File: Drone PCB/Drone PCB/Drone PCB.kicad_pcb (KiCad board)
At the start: 2 copper layers, 46 x 60 mm, 39 parts, among them J1 Conn_01x02_Socket, J2 Conn_01x02_Socket, J3 Conn_01x02_Socket, J4 Conn_01x02_Socket, J5 Conn_01x02_Socket, J6 Conn_01x02_Socket, J7 Conn_01x06_Socket, Q1 SI2302, Q2 SI2302, Q3 SI2302, Q4 SI2302, SW1 SW_SPDT, SW2 SW_Push, U1 AMS1117-3.3, U2 ATmega328P-A, U3 MPU-9250, U4 NRF24, Y1 16MHz

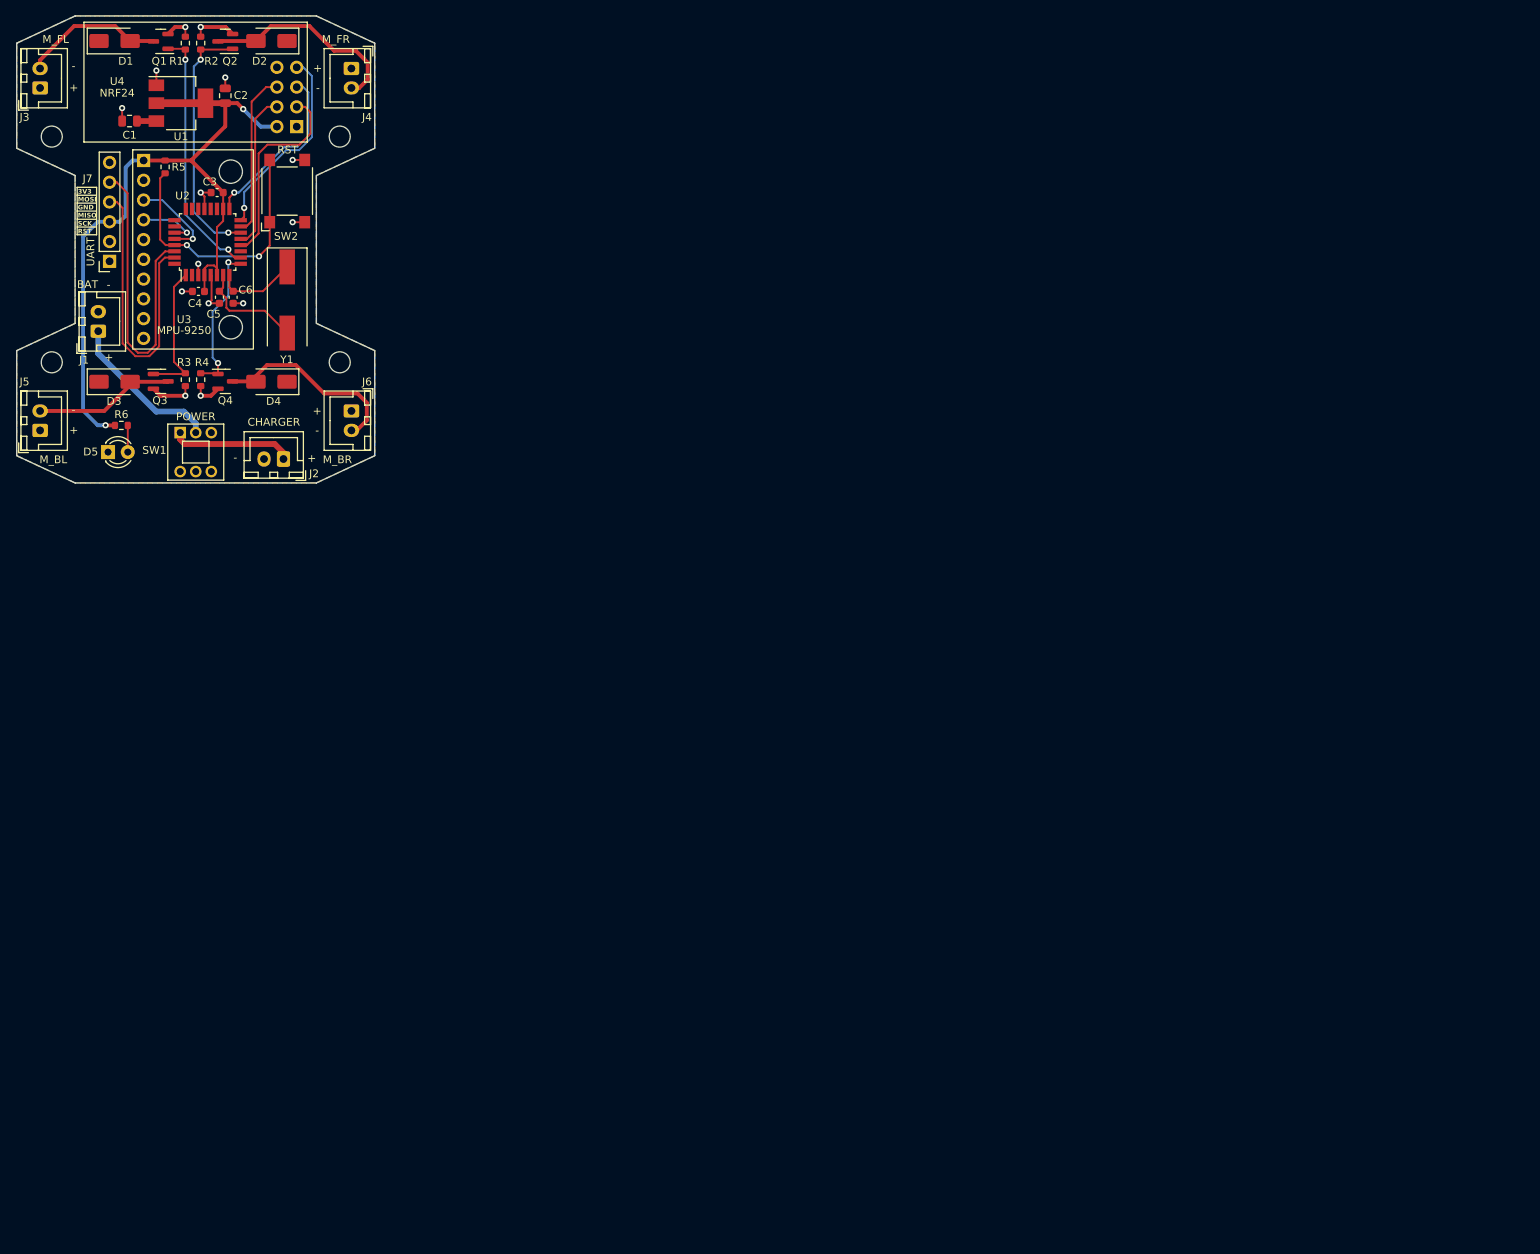
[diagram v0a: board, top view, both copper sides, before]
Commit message: Images included
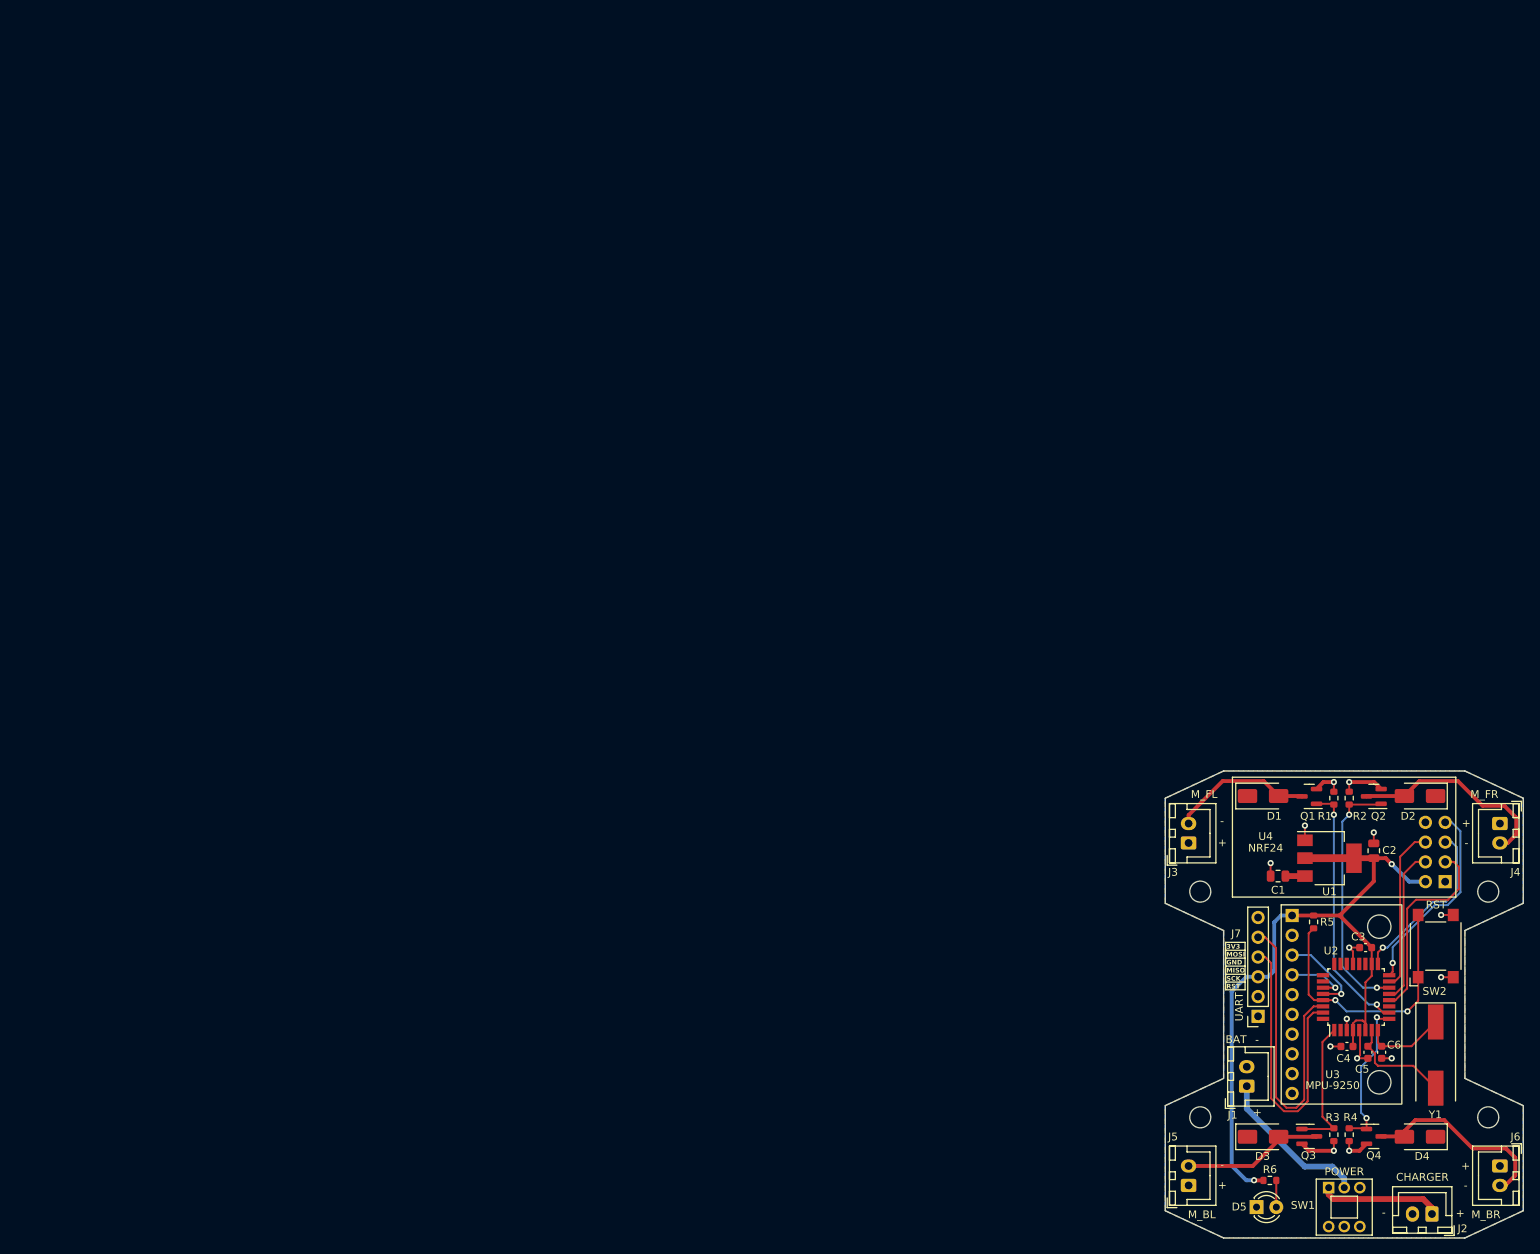
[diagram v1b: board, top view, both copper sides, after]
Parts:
- moved C2 176.6 mm to (151.4, 77.3)
- moved C3 176.6 mm to (150.3, 89.7)
- moved C4 176.6 mm to (147.9, 102.4)
- moved D5 176.6 mm to (136.3, 123.0)
- moved J1 176.6 mm to (135.0, 107.5)
- moved J7 176.6 mm to (136.5, 98.5)
- moved R5 176.6 mm to (143.6, 86.4)
- moved R6 176.6 mm to (138.0, 119.6)
- moved C1 176.6 mm to (139.1, 80.5)
- moved C5 176.6 mm to (150.6, 103.2)
- moved C6 176.6 mm to (152.4, 103.2)
- moved D1 176.6 mm to (137.1, 70.2)
- moved D2 176.6 mm to (157.3, 70.2)
- moved D3 176.6 mm to (137.1, 114.0)
- moved D4 176.6 mm to (157.3, 114.0)
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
